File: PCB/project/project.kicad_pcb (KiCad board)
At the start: 2 copper layers, 65 x 100 mm, 54 parts, among them J1 Conn_01x08_Female, J2 S1, J3 S2, J4 Conn_01x08_Female, J5 Display, J6 HC06, J7 Barrel_Jack, J8 USB_B_Micro, Q1 IRF9Z20, U1 M24C02, U2 TP4056, U3 LM1117-3.3, U4 MT3608, U5 BluePill_Connector

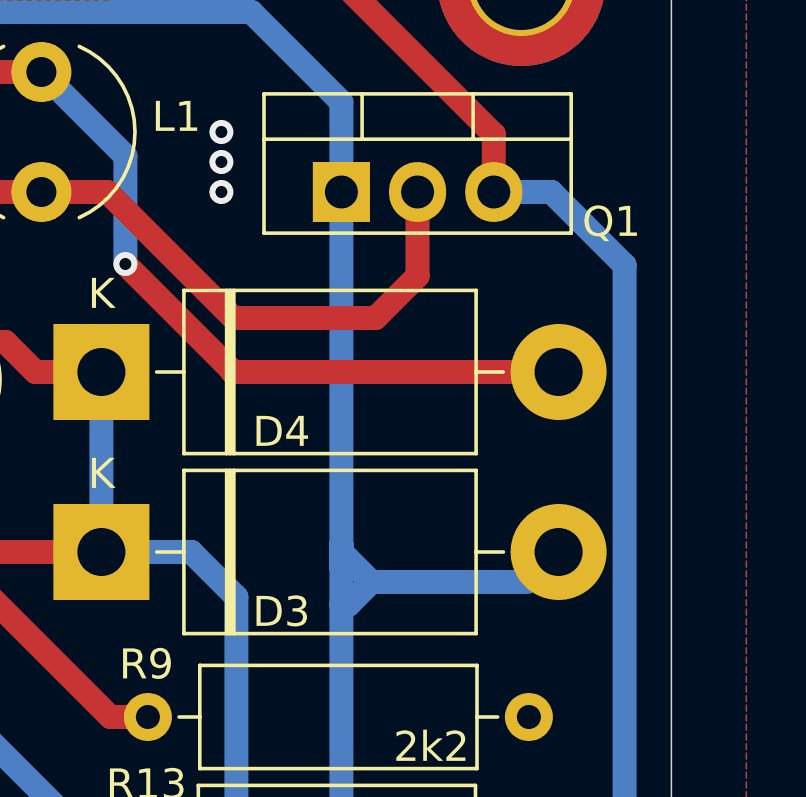
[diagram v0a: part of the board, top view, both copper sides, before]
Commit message: PCB mini bug fix
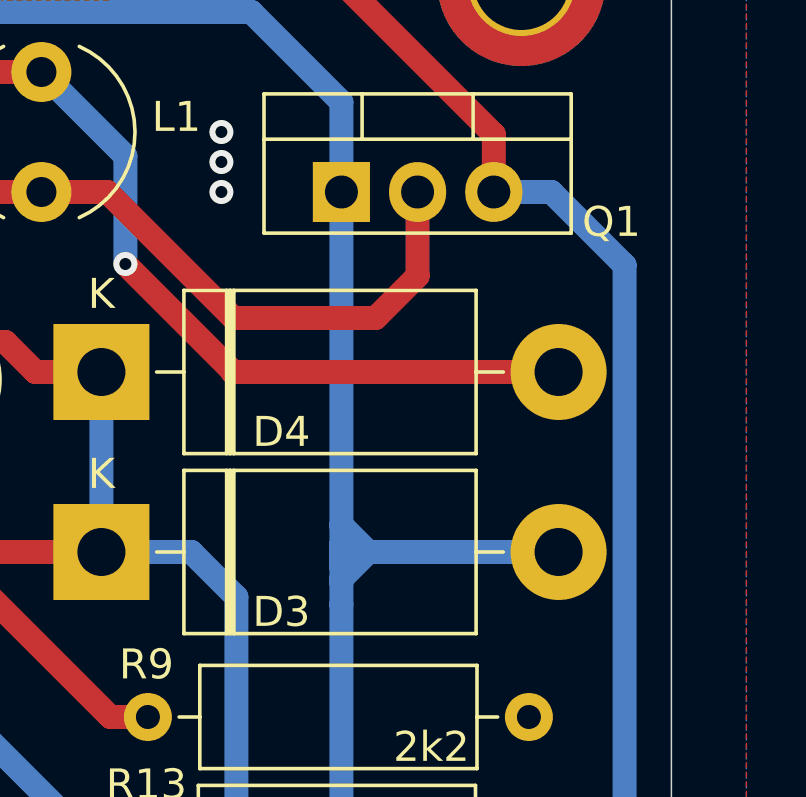
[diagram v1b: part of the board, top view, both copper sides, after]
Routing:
- net /MEASURE: track 162.9 -> 163.9 mm
